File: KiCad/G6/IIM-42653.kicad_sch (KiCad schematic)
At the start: 8 parts, among them U13 IIM-42653, U14 IIM-42653

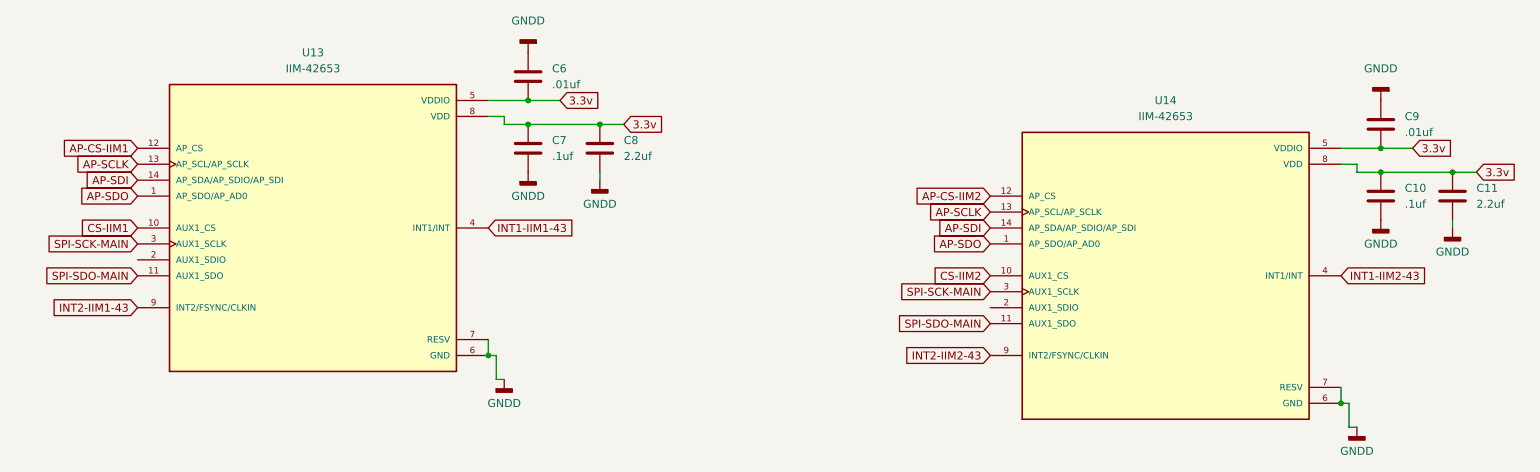
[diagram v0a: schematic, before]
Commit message: uhhhh im confused gang
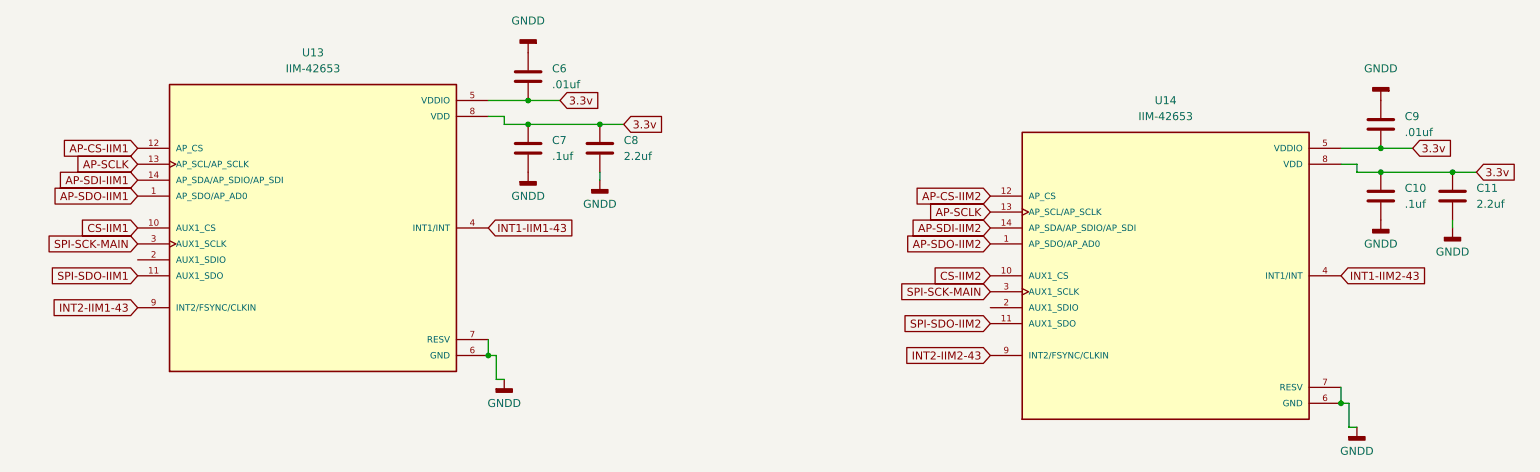
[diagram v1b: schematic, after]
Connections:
- net AP-SDI renamed AP-SDI-IIM1
- net AP-SDI-IIM1: no longer U14.14 (AP_SDA/AP_SDIO/AP_SDI)
- net AP-SDO renamed AP-SDO-IIM1
- net AP-SDO-IIM1: no longer U14.1 (AP_SDO/AP_AD0)
- net SPI-SDO-MAIN renamed SPI-SDO-IIM1
- net SPI-SDO-IIM1: no longer U14.11 (AUX1_SDO)
- new net AP-SDI-IIM2: U14.14 (AP_SDA/AP_SDIO/AP_SDI)
- new net AP-SDO-IIM2: U14.1 (AP_SDO/AP_AD0)
- new net SPI-SDO-IIM2: U14.11 (AUX1_SDO)
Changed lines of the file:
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@@
 		)
 	)
-	(global_label "AP-SDI"
+	(global_label "AP-SDI-IIM1"
 		(shape input)
 		(at 44.45 92.71 180)
@@
 		)
 		(property "Intersheetrefs" "${INTERSHEET_REFS}"
-			(at 34.4495 92.71 0)
+			(at 29.0066 92.71 0)
 			(effects
 				(font
@@
 		)
 	)
-	(global_label "AP-SDO"
+	(global_label "AP-SDO-IIM1"
 		(shape input)
 		(at 44.45 95.25 180)
@@
 		)
 		(property "Intersheetrefs" "${INTERSHEET_REFS}"
-			(at 33.7238 95.25 0)
+			(at 28.2809 95.25 0)
 			(effects
 				(font
@@
 		)
 	)
-	(global_label "SPI-SDO-MAIN"
+	(global_label "SPI-SDO-IIM1"
 		(shape input)
 		(at 44.45 107.95 180)
@@
 		)
 		(property "Intersheetrefs" "${INTERSHEET_REFS}"
-			(at 26.9504 107.95 0)
+			(at 27.5552 107.95 0)
 			(effects
 				(font
@@
 		)
 	)
-	(global_label "AP-SDI"
+	(global_label "AP-SDI-IIM2"
 		(shape input)
 		(at 180.34 100.33 180)
@@
 		)
 		(property "Intersheetrefs" "${INTERSHEET_REFS}"
-			(at 170.3395 100.33 0)
+			(at 164.8966 100.33 0)
 			(effects
 				(font
@@
 		)
 	)
-	(global_label "AP-SDO"
+	(global_label "AP-SDO-IIM2"
 		(shape input)
 		(at 180.34 102.87 180)
@@
 		)
 		(property "Intersheetrefs" "${INTERSHEET_REFS}"
-			(at 169.6138 102.87 0)
-			(effects
-				(font
-					(size 1.27 1.27)
-				)
-				(justify right)
-				(hide yes)
-			)
-		)
-	)
-	(global_label "SPI-SDO-MAIN"
+			(at 164.1709 102.87 0)
+			(effects
+				(font
+					(size 1.27 1.27)
+				)
+				(justify right)
+				(hide yes)
+			)
+		)
+	)
+	(global_label "SPI-SDO-IIM2"
 		(shape input)
 		(at 180.34 115.57 180)
@@
 		)
 		(property "Intersheetrefs" "${INTERSHEET_REFS}"
-			(at 162.8404 115.57 0)
-			(effects
-				(font
+			(at 163.4452 115.57 0)
+			(effects
+				(font
